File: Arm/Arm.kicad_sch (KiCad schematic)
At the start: 55 parts, among them J10 SparkMAX XT60 F, J11 CAN OUT, J12 SparkMAX XT60 F, J13 SparkMAX XT60 F, J14 Encoder 0, J2 Encoder Bundle, J3 CAN IN, J4 5V Swtich Power, J5 Power IN XT60 M, J6 SparkMAX XT60 F, J7 Power OUT XT60 F, J8 Lynx, J9 CANBUS, M1 Fan, U4 TJA1051T, U5 TJA1051T, U7 RASPBERRY_PI_4B_4GB

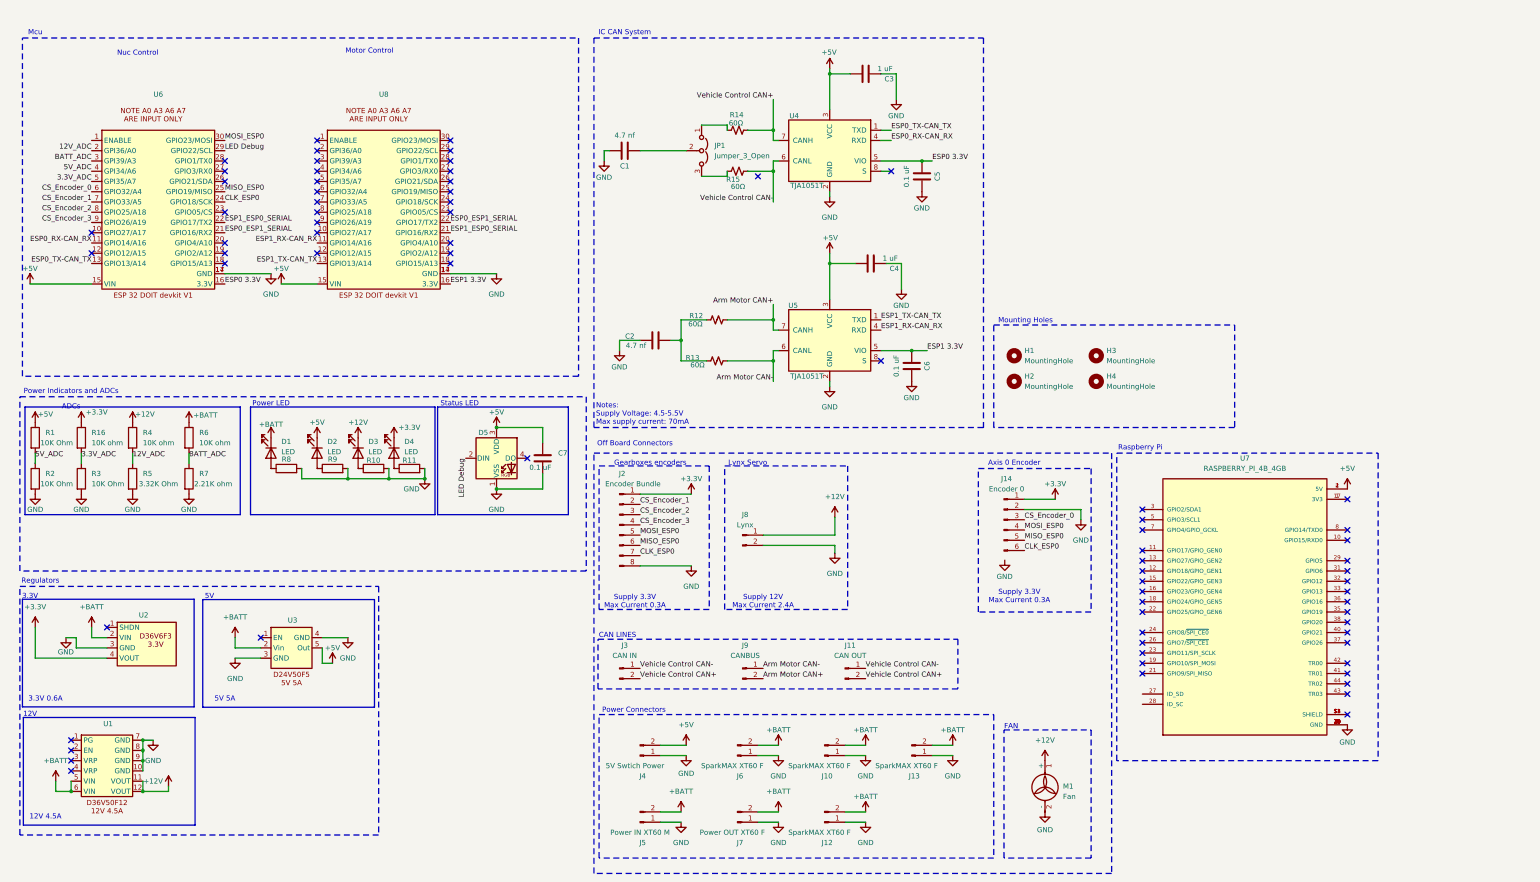
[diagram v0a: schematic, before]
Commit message: PCB Layout....
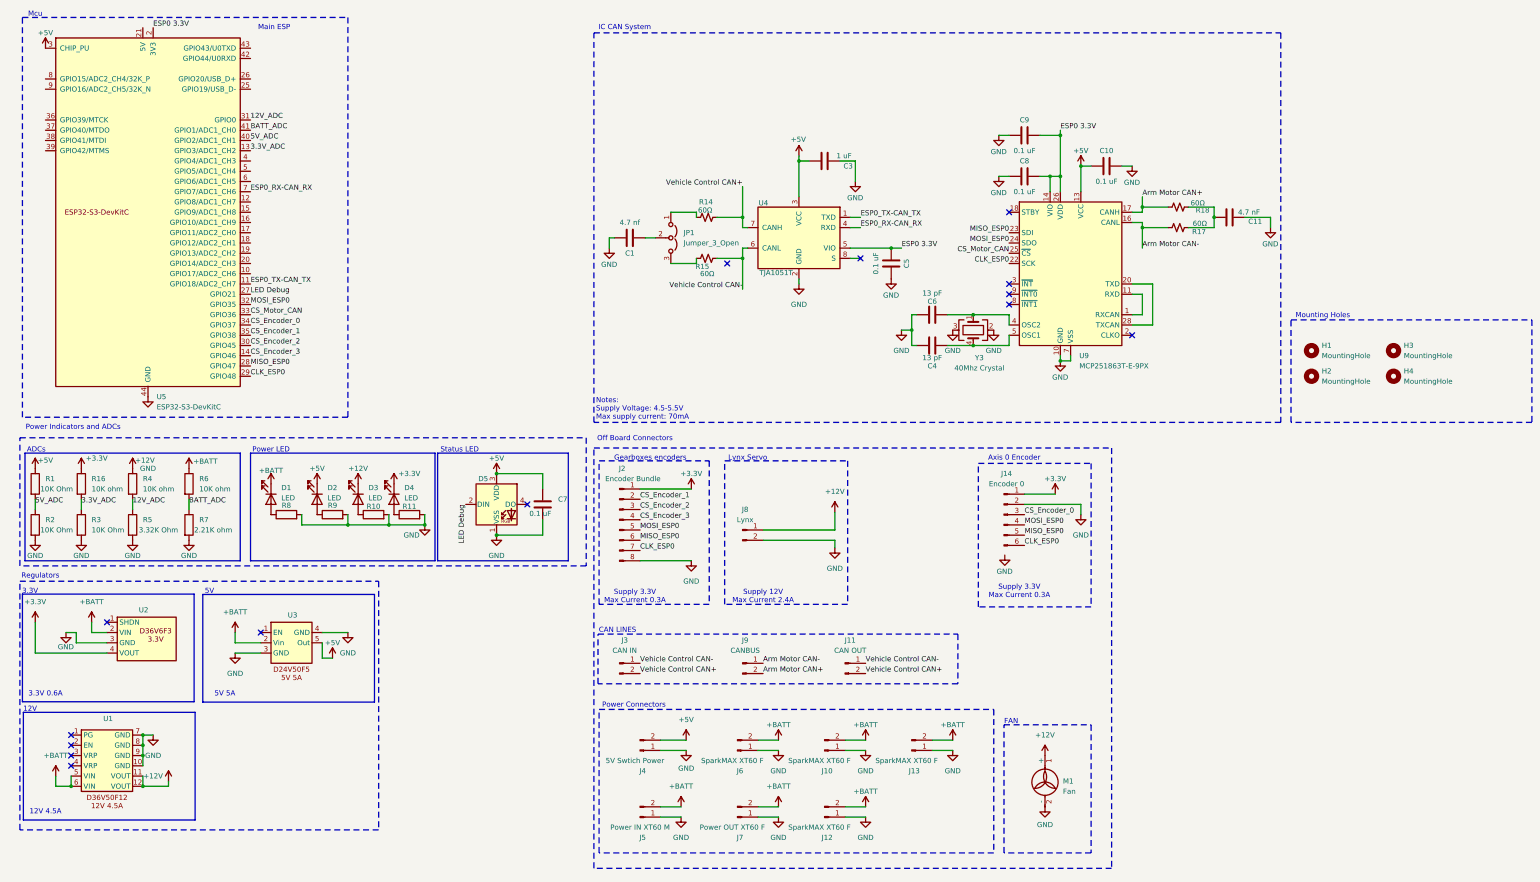
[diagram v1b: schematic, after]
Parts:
- removed C2: 4.7 nf, Capacitor_SMD:C_0603_1608Metric_Pad1.08x0.95mm_HandSolder, symbol Device:C
- removed R12, R13: 60Ω, Resistor_SMD:R_0603_1608Metric_Pad0.98x0.95mm_HandSolder, symbol Device:R_Small_US
- removed U5: TJA1051T, Package_SO:SOIC-8_3.9x4.9mm_P1.27mm, symbol Interface_CAN_LIN:TJA1051T-3
- removed U6, U8: ~, ESP 32 DOIT devkit V1:esp32_devkit_v1_doit, symbol ESP 32 DOIT devkit V1:ESP32_DOIT_devkit_V1
- removed U7: RASPBERRY_PI_4B_4GB, RASPBERRY_PI_4B_4GB:MODULE_RASPBERRY_PI_4B_4GB, symbol RASPBERRY_PI_4B_4GB:RASPBERRY_PI_4B_4GB
- added C10, C8, C9: 0.1 uF, Capacitor_SMD:C_0603_1608Metric_Pad1.08x0.95mm_HandSolder, symbol Device:C
- added C11: 4.7 nF, Capacitor_SMD:C_0603_1608Metric_Pad1.08x0.95mm_HandSolder, symbol Device:C
- added R17, R18: 60Ω, Resistor_SMD:R_0603_1608Metric_Pad0.98x0.95mm_HandSolder, symbol Device:R_Small_US
- added U5: ESP32-S3-DevKitC, Astra Lib:ESP32-S3-DevKitC, symbol ESP32-S3-DevkitC:ESP32-S3-DevKitC
- added U9: MCP251863T-E-9PX, Package_DFN_QFN:VQFN-28-1EP_5x5mm_P0.5mm_EP3.25x3.25mm, symbol Interface_CAN_LIN:MCP251863T-E-9PX
- added Y3: 40Mhz Crystal, Crystal:Crystal_SMD_3225-4Pin_3.2x2.5mm, symbol Device:Crystal_GND23
- C4: value 1 uF -> 13 pF
- C6: value 0.1 uF -> 13 pF
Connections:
- net +5V: now also C10.2, U5.3 (CHIP_PU), U9.13 (VCC); no longer C4.1
- net 12V_ADC: now also U5.31 (GPIO0)
- net 3.3V_ADC: now also U5.13 (GPIO3/ADC1_CH2)
- net 5V_ADC: now also U5.40 (GPIO2/ADC1_CH1)
- net Arm Motor CAN+: now also R18.2, U9.17 (CANH)
- net Arm Motor CAN-: now also R17.1, U9.16 (CANL)
- net BATT_ADC: now also U5.41 (GPIO1/ADC1_CH0)
- net CLK_ESP0: now also U5.29 (GPIO48), U9.22 (SCK)
- net CS_Encoder_0: now also U5.34 (GPIO37)
- net CS_Encoder_1: now also U5.35 (GPIO38)
- net CS_Encoder_2: now also U5.30 (GPIO45)
- net CS_Encoder_3: now also U5.14 (GPIO46)
- net ESP0 3.3V: now also C8.1, C9.1, U5.1 (3V3), U5.2 (3V3), U9.14 (VIO), U9.26 (VDD)
- net ESP0_RX-CAN_RX: now also U5.7 (GPIO7/ADC1_CH6)
- net ESP0_TX-CAN_TX: now also U5.11 (GPIO18/ADC2_CH7)
- net GND: now also C4.1, C10.1, C11.1, C8.2, C9.2, U5.22 (GND), U5.23 (GND), U5.24 (GND), U5.44 (GND), U9.10 (GND), U9.7 (VSS), Y3.2, Y3.3; no longer C4.2
- net LED Debug: now also U5.27 (GPIO21)
- net MISO_ESP0: now also U5.28 (GPIO47), U9.23 (SDI)
- net MOSI_ESP0: now also U5.32 (GPIO35), U9.24 (SDO)
- net ESP1 3.3V: no longer names the net of C6.2
- net ESP1 3.3V: now also U9.4 (OSC2), Y3.1
- new net: C4.2, U9.5 (OSC1), Y3.4
- new net: C11.2, R17.2, R18.1
- new net: U9.1 (RXCAN), U9.11 (RXD)
- new net: U9.20 (TXD), U9.28 (TXCAN)
- new net CS_Motor_CAN: U5.33 (GPIO36), U9.25 (~{CS})
- no-connect marks 73 -> 14
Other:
- note added: "Main ESP"
- note removed: "Motor Control"
- note removed: "Nuc Control"
- note removed: "Raspberry Pi"
- moved on the sheet: C1, C3, C5, C7, D1, D2, D3, D4, D5, H1, H2, H3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
